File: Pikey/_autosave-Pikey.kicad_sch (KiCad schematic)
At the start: 58 parts, among them J1 DX07P024AJ1R1500, J2 Conn_01x03, J3 Micro_SD_Card_Det2, SW1 CK_KMS2xxG, SW2 CK_KMS2xxG, U1 RP2350B, U2 NCP1117-3.3_SOT223, U3 W25Q128JVS, Y1 ABM8-272-T3

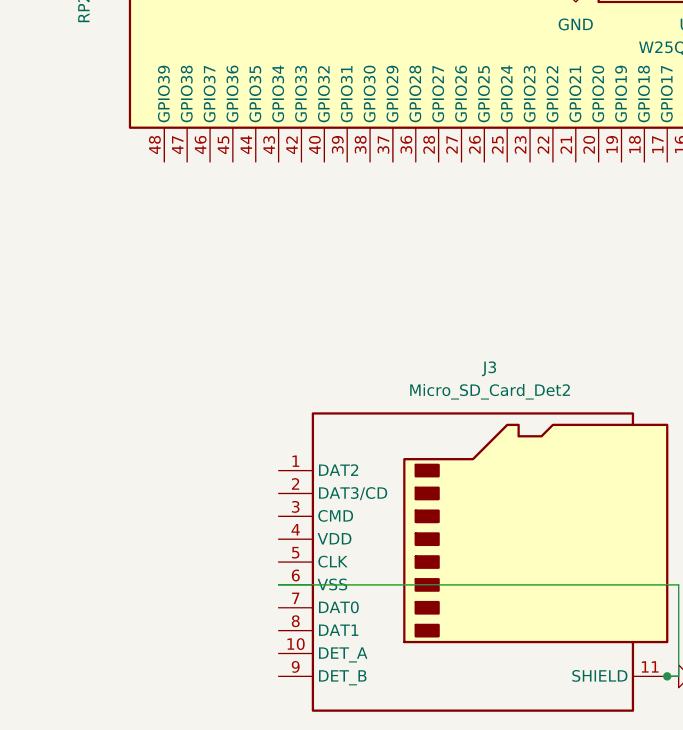
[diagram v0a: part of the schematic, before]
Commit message: Sunday 12th April update
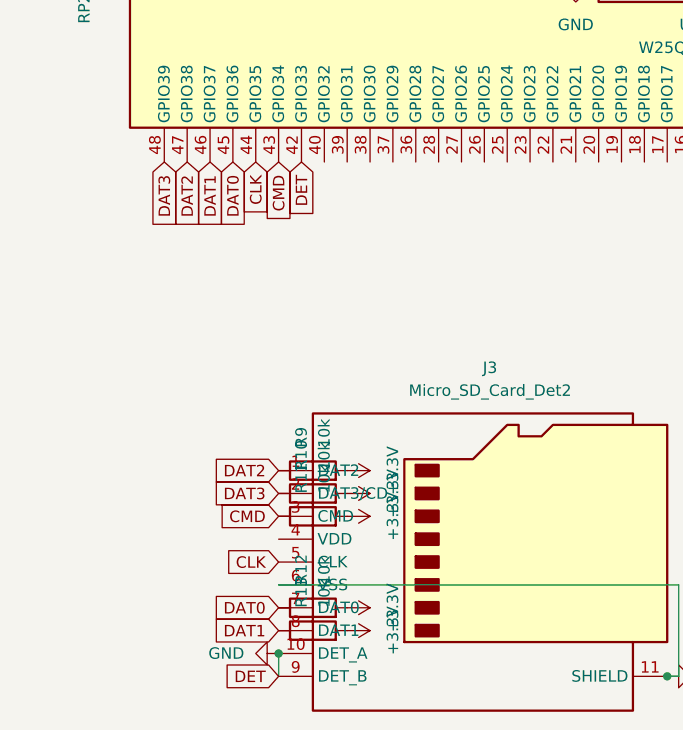
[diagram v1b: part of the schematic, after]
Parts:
- added R10, R11, R12, R13, R9: 10k, Resistor_SMD:R_0201_0603Metric, symbol Device:R
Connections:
- net +3.3V: now also R10.2, R11.2, R12.2, R13.2, R9.2
- net GND: now also J3.10 (DET_A), J3.9 (DET_B), U1.42 (GPIO33)
- net DAT2: now reaches J3.1 (DAT2)
- net DAT2: now also U1.47 (GPIO38), R9.1
- net DAT3: now reaches J3.2 (DAT3/CD)
- net DAT3: now also U1.48 (GPIO39), R10.1
- net CMD: now reaches J3.3 (CMD)
- net CMD: now also U1.43 (GPIO34), R11.1
- net CLK: now reaches J3.5 (CLK)
- net CLK: now also U1.44 (GPIO35)
- net DAT0: now reaches J3.7 (DAT0)
- net DAT0: now also U1.45 (GPIO36), R12.1
- net DAT1: now reaches J3.8 (DAT1)
- net DAT1: now also U1.46 (GPIO37), R13.1
